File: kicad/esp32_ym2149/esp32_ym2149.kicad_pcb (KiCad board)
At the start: 2 copper layers, 26 parts, among them IC1 LM386, J1 5V_OUT, J2 3V3_OUT, U1 LM1086-5, U2 LM1086-3.3

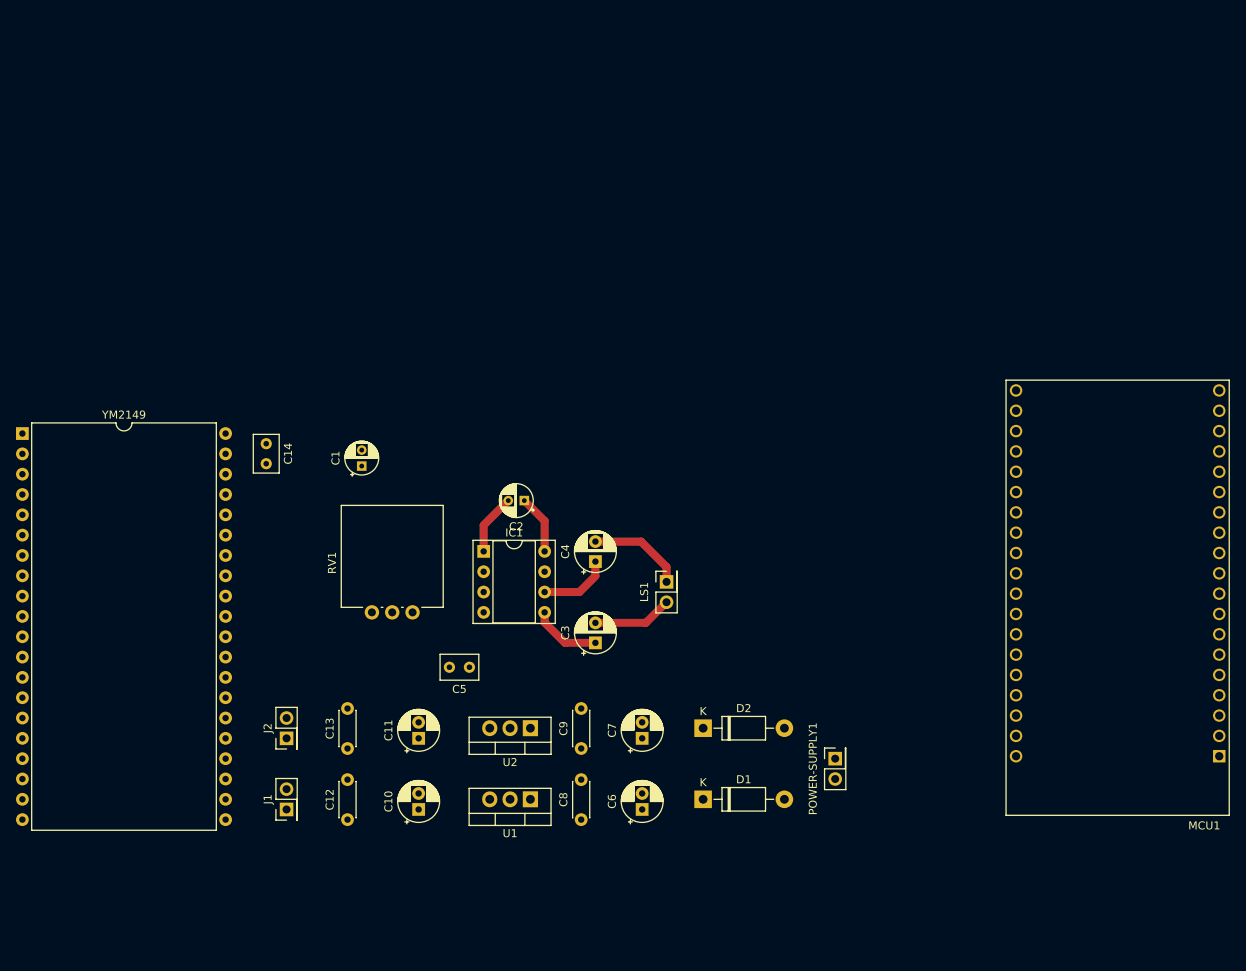
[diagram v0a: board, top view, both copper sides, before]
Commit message: new symbols and footprints added
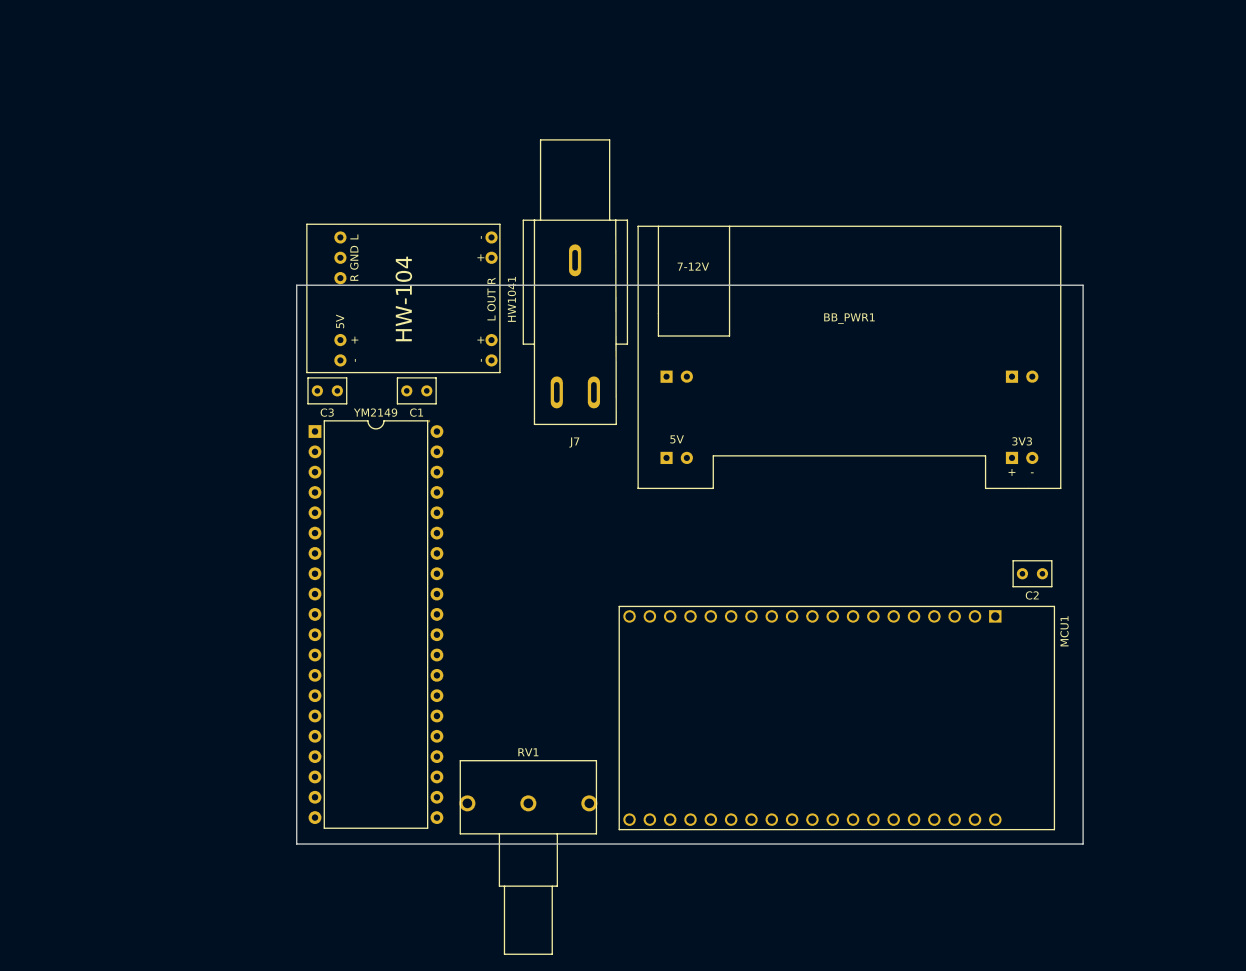
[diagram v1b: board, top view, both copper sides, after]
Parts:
- removed C10, C11, C6, C7: 100uF, Capacitor_THT:CP_Radial_D5.0mm_P2.00mm
- removed C12, C13, C8, C9: 100nF, Capacitor_THT:C_Disc_D4.3mm_W1.9mm_P5.00mm
- removed the C2 at (141.7, 83.6)
- removed the C3 at (150.6, 101.3)
- removed C4: 220uF, 16V, Capacitor_THT:CP_Radial_D5.0mm_P2.50mm
- removed D1, D2: 1N4004, Diode_THT:D_DO-41_SOD81_P10.16mm_Horizontal
- removed IC1: LM386, Package_DIP:DIP-8_W7.62mm_Socket
- removed J1: 5V_OUT, Connector_PinHeader_2.54mm:PinHeader_2x01_P2.54mm_Vertical
- removed J2: 3V3_OUT, Connector_PinHeader_2.54mm:PinHeader_2x01_P2.54mm_Vertical
- removed LS1: 8 Ohm 1W, Connector_PinSocket_2.54mm:PinSocket_2x01_P2.54mm_Vertical
- removed POWER-SUPPLY1: 6-12V, Connector_PinSocket_2.54mm:PinSocket_2x01_P2.54mm_Vertical
- removed U1: LM1086-5, Package_TO_SOT_THT:TO-220-3_Vertical
- removed U2: LM1086-3.3, Package_TO_SOT_THT:TO-220-3_Vertical
- added BB_PWR1: BreadboardPowerSupply, dl1xy:Breadboard_Powersupply_3V3_5V, F.Cu at (182.4, 60.2)
- added HW1041: HW-104_Board, dl1xy:HW-104 Board, F.Cu at (140.7, 58.4)
- added J7: AudioJack3, dl1xy:AudioJack 6.5mm, F.Cu at (148.1, 76.7)
- C1: value 10uF, 16V -> 10nF; footprint Capacitor_THT:CP_Radial_D4.0mm_P2.00mm -> Capacitor_THT:C_Rect_L4.6mm_W3.0mm_P2.50mm_MKS02_FKP02
- MCU1: footprint MODULE_ESP32-DEVKITC-32D -> ESP32_Dev:MODULE_ESP32-DEVKITC-32D
- RV1: value 10K -> 10 kOhm; footprint Potentiometer_THT:Potentiometer_Vishay_148-149_Single_Vertical -> dl1xy:ALPHA POT 16 RV16
- YM2149: value YM2149 -> Yamaha_YM2149; footprint Package_DIP:DIP-40_W25.4mm -> Package_DIP:DIP-40_W15.24mm
- moved C2 72.6 mm to (206.5, 92.7)
- moved MCU1 38.1 mm to (180.8, 110.7), turned to 270 degrees
- moved YM2149 36.6 mm to (115.6, 74.9)
- moved RV1 23.8 mm to (142.2, 116.5), turned to 0 degrees
- moved C1 12.4 mm to (129.5, 69.8), turned to 180 degrees
- moved C3 11.1 mm to (118.4, 69.8), turned to 180 degrees
- renumbered C5 to C2, C14 to C3
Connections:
- net +3V3 renamed +3.3V
- C1 pad 1: AUDIO_CH_A -> GNDREF
- C1 pad 2: Net-(C1-Pad2) -> +5V
- MCU1 pad 10: DA5 -> DA6
- MCU1 pad 11: DA4 -> DA5
- MCU1 pad 12: BDIR -> DA4
- MCU1 pad 13: BC1 -> BDIR
- MCU1 pad 15: Net-(MCU1-Pad15) -> BC1
- MCU1 pad 26: GNDREF -> Net-(MCU1-Pad26)
- MCU1 pad 30: DA2 -> Net-(MCU1-Pad30)
- MCU1 pad 31: DA1 -> DA2
- MCU1 pad 32: DA0 -> DA1
- MCU1 pad 33: Net-(MCU1-Pad33) -> DA0
- MCU1 pad 34: RESET -> Net-(MCU1-Pad34)
- MCU1 pad 35: CLOCK -> RESET
- MCU1 pad 36: Net-(MCU1-Pad36) -> CLOCK
- MCU1 pad 8: DA7 -> Net-(MCU1-Pad8)
- MCU1 pad 9: DA6 -> DA7
- RV1 pad 2: Net-(C1-Pad2) -> Net-(HW1041-Pad1)
- RV1 pad 3: Net-(IC1-Pad3) -> Net-(RV1-Pad3)
- YM2149 pad 3: AUDIO_CH_A -> Net-(RV1-Pad3)
- YM2149 pad 38: AUDIO_CH_A -> Net-(RV1-Pad3)
- YM2149 pad 4: AUDIO_CH_A -> Net-(RV1-Pad3)
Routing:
- net GNDREF: track 13.2 -> 0.00 mm
- net Net-(C3-Pad2): track 9.96 -> 0.00 mm
- net +5V: track 8.98 -> 0.06 mm
- net Net-(C3-Pad1): track 8.67 -> 0.00 mm
- net Net-(C2-Pad2): track 7.63 -> 0.00 mm
- net Net-(C2-Pad1): track 7.40 -> 0.00 mm
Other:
- board outline added: 98.3 x 69.8 mm
- net class Power added: clearance 0.3, trace_width 0.3, via_dia 1, via_drill 0.5

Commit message: layout changes
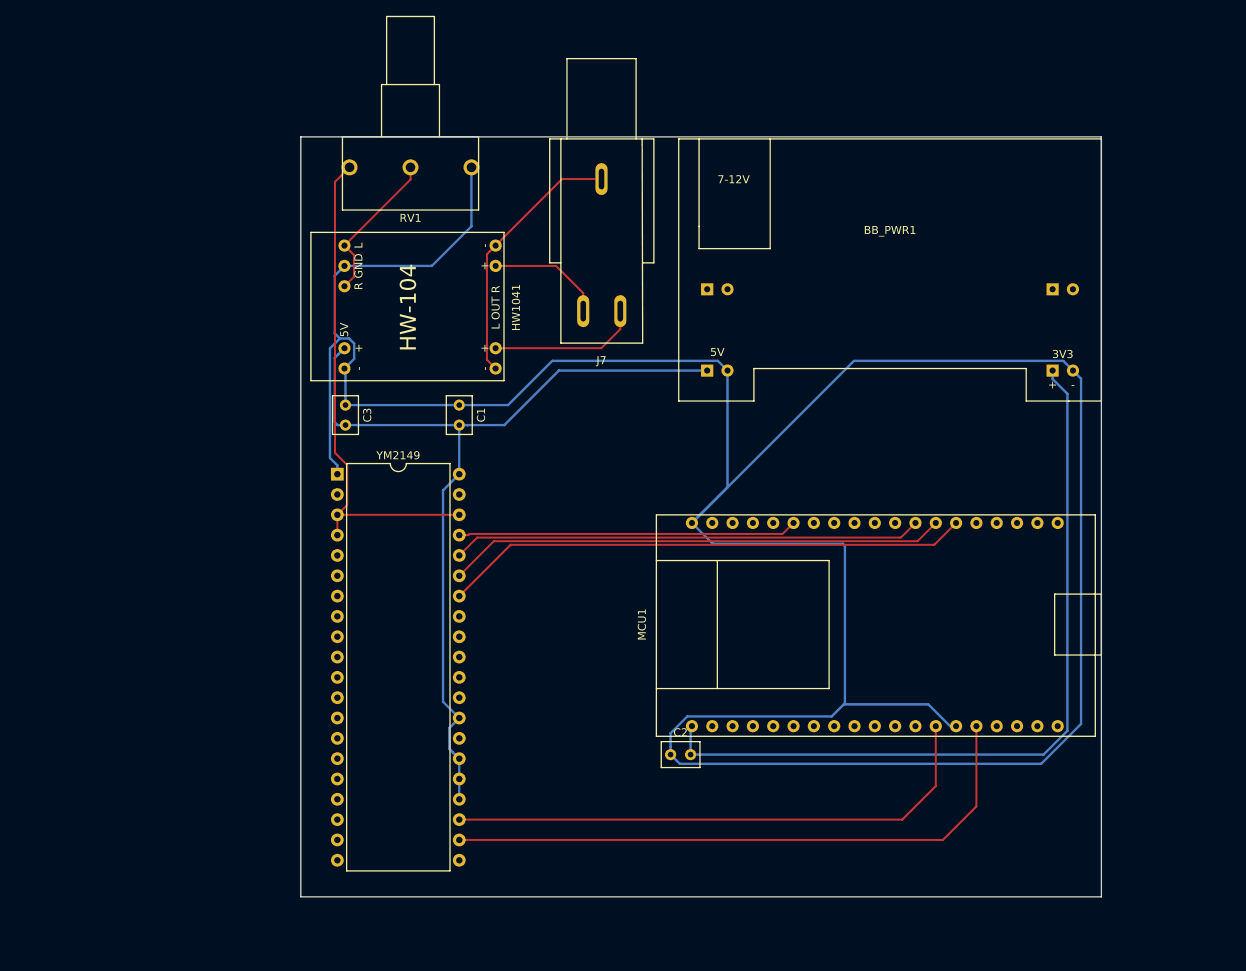
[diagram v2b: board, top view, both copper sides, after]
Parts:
- MCU1: footprint ESP32_Dev:MODULE_ESP32-DEVKITC-32D -> dl1xy:ESP32-WROOM-Devkit
- moved RV1 71.1 mm to (127.5, 46.9), turned to 180 degrees
- moved C2 51.7 mm to (160.0, 115.3), turned to 0 degrees
- moved MCU1 28.9 mm to (154.4, 99.1), turned to 90 degrees
- moved BB_PWR1 12.0 mm to (187.5, 49.3)
- moved J7 10.7 mm to (151.4, 66.5)
- moved YM2149 6.02 mm to (118.4, 80.3)
- moved C1 4.44 mm to (133.6, 71.6), turned to 270 degrees
- moved C3 2.05 mm to (119.4, 71.6), turned to 270 degrees
- moved HW1041 1.14 mm to (141.2, 59.4)
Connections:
- MCU1 pad 13: BDIR -> RESET
- MCU1 pad 15: BC1 -> CLOCK
- MCU1 pad 25: DA3 -> DA0
- MCU1 pad 31: DA2 -> DA1
- MCU1 pad 32: DA1 -> DA2
- MCU1 pad 33: DA0 -> DA3
- MCU1 pad 35: RESET -> Net-(MCU1-Pad35)
- MCU1 pad 36: CLOCK -> Net-(MCU1-Pad36)
- MCU1 pad 7: Net-(MCU1-Pad7) -> BDIR
- MCU1 pad 8: Net-(MCU1-Pad8) -> BC1
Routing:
- net GNDREF: track 0.00 -> 370.8 mm
- net +5V: track 0.06 -> 108.8 mm
- net +3.3V: track 0.00 -> 97.8 mm
- net CLOCK: track 0.00 -> 76.4 mm
- net RESET: track 0.00 -> 68.8 mm
- net DA3: track 0.00 -> 65.9 mm
- net Net-(RV1-Pad3): track 0.00 -> 63.1 mm
- net DA2: track 0.00 -> 62.3 mm
- net DA1: track 0.00 -> 58.7 mm
- net DA0: track 0.00 -> 42.4 mm
- net Net-(HW1041-Pad6): track 0.00 -> 33.0 mm
- net Net-(HW1041-Pad1): track 0.00 -> 19.3 mm
- net Net-(HW1041-Pad8): track 0.00 -> 18.8 mm
- net Net-(HW1041-Pad7): track 0.00 -> 14.6 mm
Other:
- board size 98.3 x 69.8 mm -> 100.1 x 95 mm
